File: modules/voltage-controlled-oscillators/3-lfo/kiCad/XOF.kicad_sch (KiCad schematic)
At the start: 78 parts, among them Q1 2N3904, Q2 2N3904, SW1 SW_SPDT, U1 TL074, U2 TL074

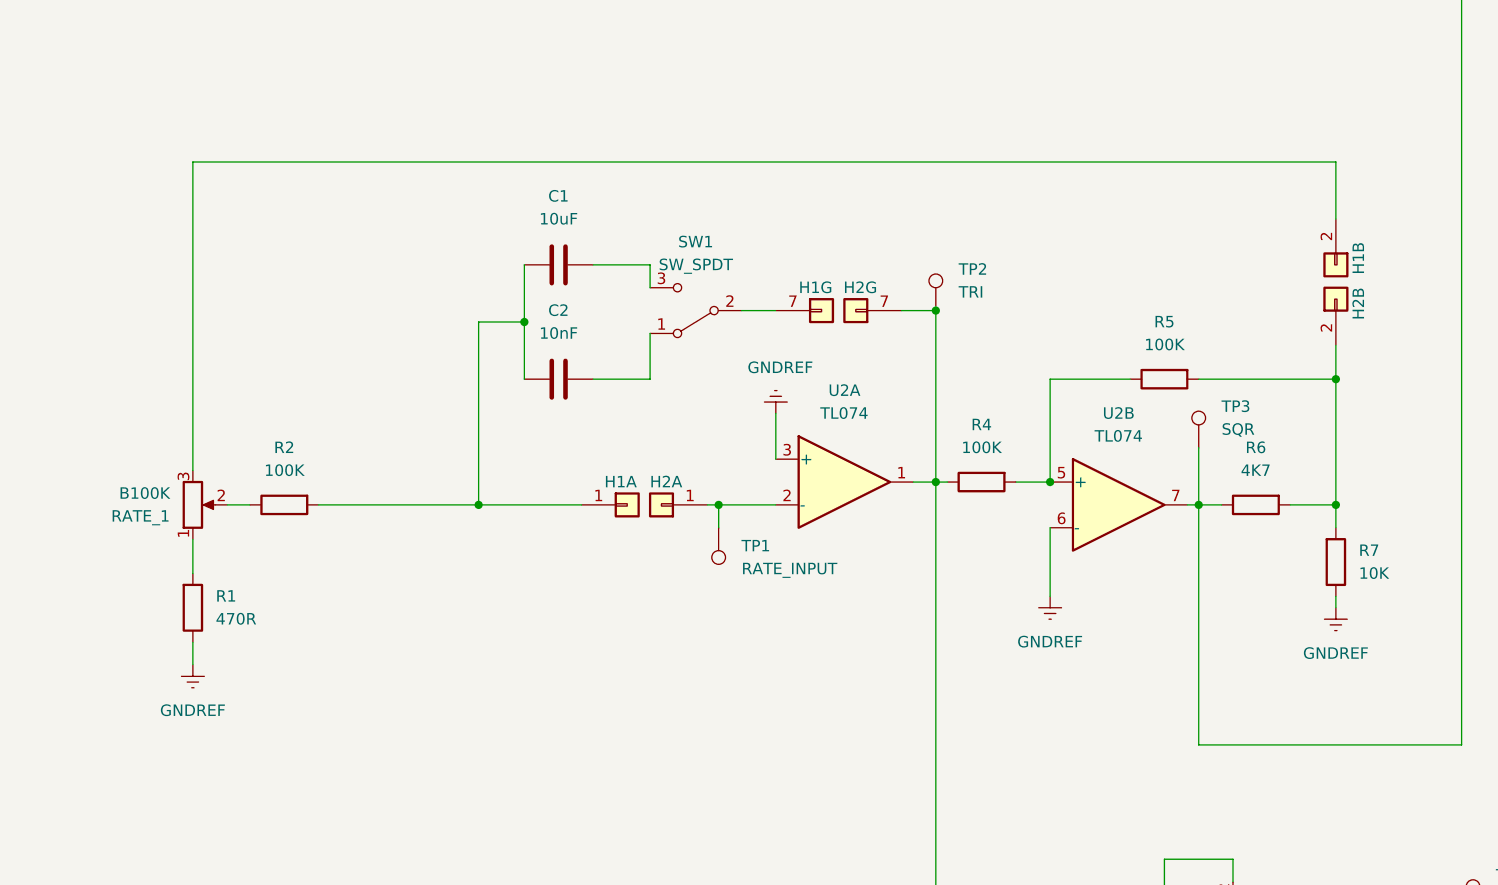
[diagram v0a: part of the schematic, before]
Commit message: update components, PCB 3320 and design
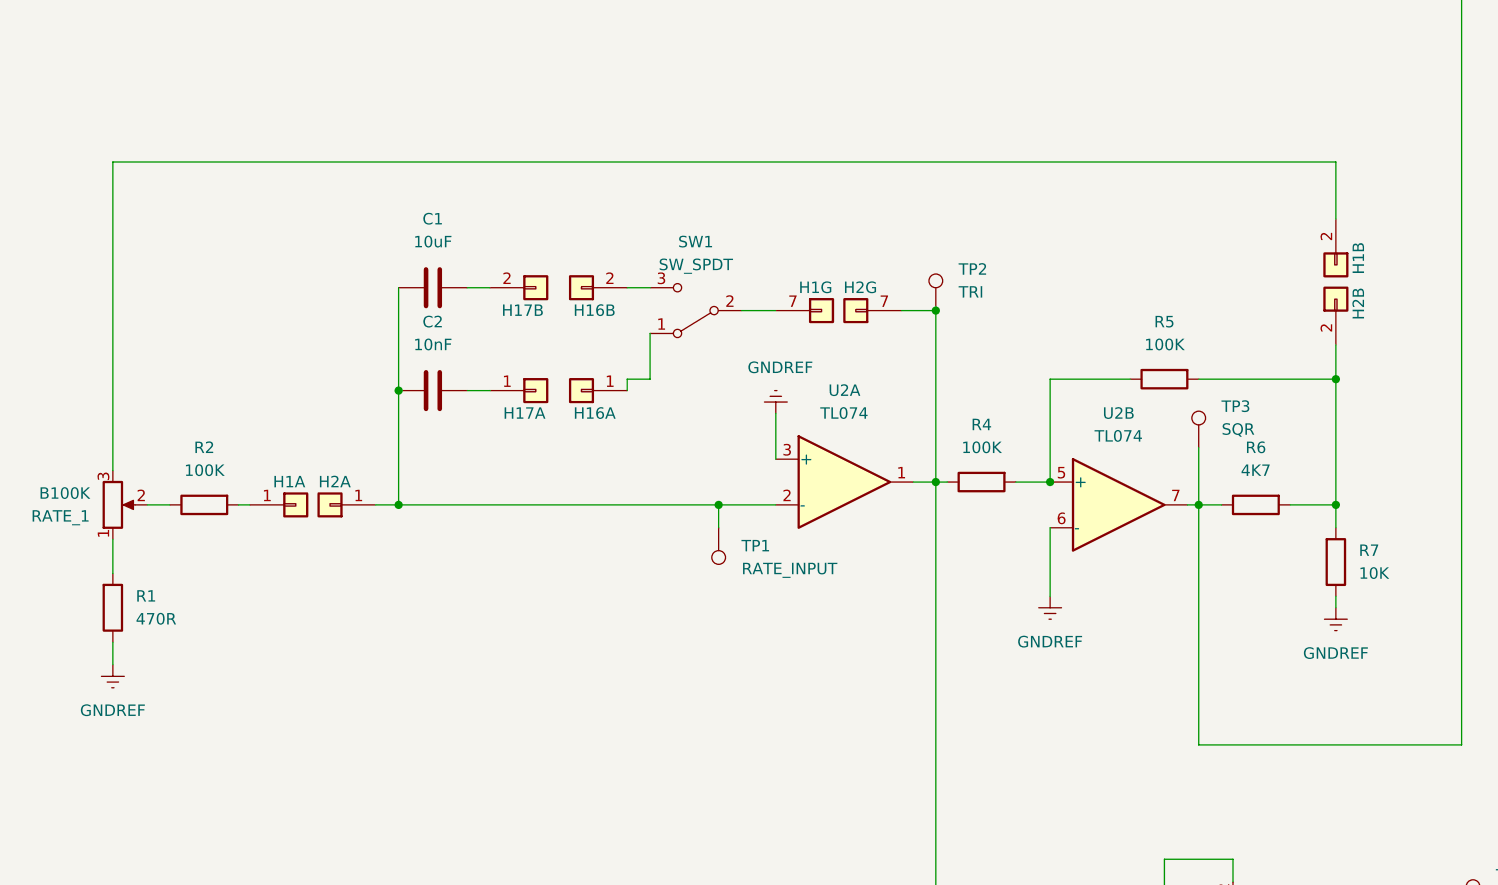
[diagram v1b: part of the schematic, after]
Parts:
- added H16: PinHeader_01x02, Synth:PinHeader_1x02_P2.54mm_Vertical, symbol synth:PinHeader_01x02
- added H17: PinSocket_01x02, Synth:PinSocket_1x02_P2.54mm_Vertical, symbol synth:PinSocket_01x02
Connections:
- net at H1.1 (Pin_1), R2.1: no longer C1.1, C2.1
- net at H2.1 (Pin_3), TP1.1, U2.2 (-): now also C1.1, C2.1
- net at C1.2: now also H17.2 (Pin_2); no longer SW1.3 (C)
- net at SW1.1 (A): now also H16.1 (Pin_1); no longer C2.2
- new net: H16.2 (Pin_2), SW1.3 (C)
- new net: C2.2, H17.1 (Pin_1)
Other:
- moved on the sheet: C1, C2, R1, R2, RATE_1
